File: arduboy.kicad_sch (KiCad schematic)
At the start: 59 parts, among them J1 Conn_01x06_Pin, J2 Conn_01x01_Pin, J3 Conn_01x01_Pin, J4 Conn_01x01_Pin, J5 Conn_01x01_Pin, J6 Conn_01x01_Pin, J7 Conn_01x01_Pin, SW1 POWER, SW2 LEFT, SW3 UP, SW4 DOWN, SW5 RIGHT, SW6 A, SW7 B, SW8 RESET, U1 ATmega32U4-A, U2 USBLC6-2SC6, U3 MCP73831-2-OT, U4 W25Q128JVS, Y1 16MHz

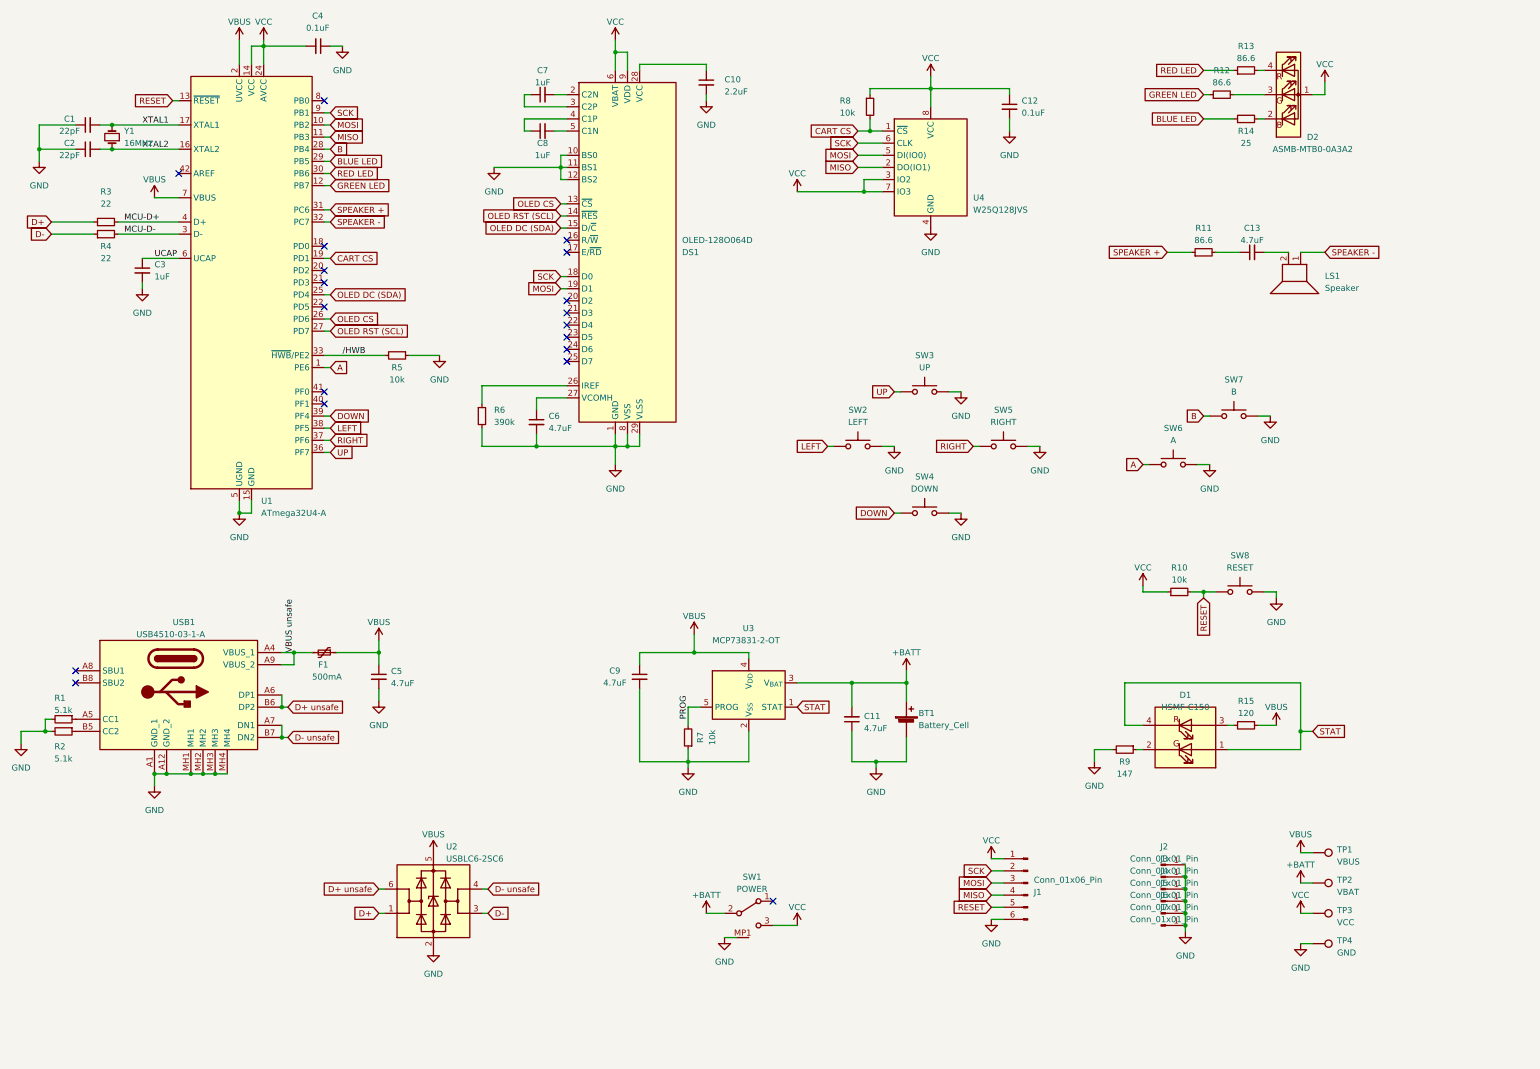
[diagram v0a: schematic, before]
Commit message: Add back silkscreen
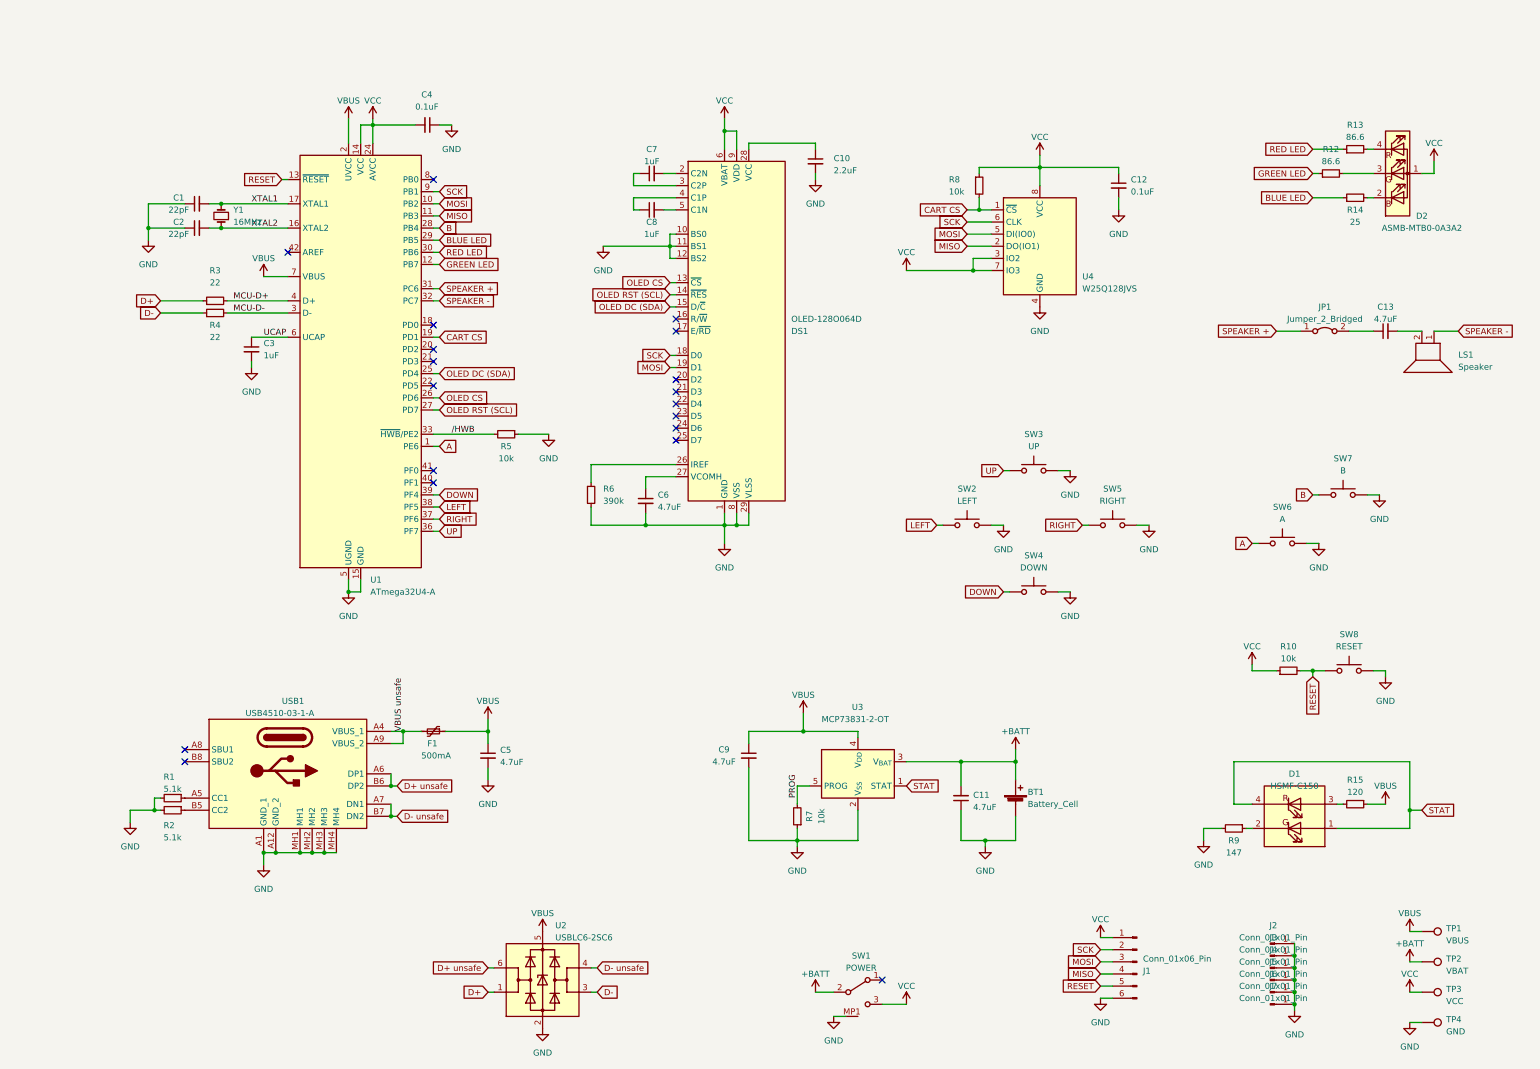
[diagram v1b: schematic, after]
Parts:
- removed R11: 86.6, arduboy:R_1210_3225Metric_Pad1.30x2.65mm_HandSolder with ref under the component, symbol Device:R_Small
- added JP1: Jumper_2_Bridged, arduboy:Jumper for SMD 1210 bridged, symbol Jumper:Jumper_2_Bridged
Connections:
- net SPEAKER +: now also JP1.1 (A)
- net at C13.1: now also JP1.2 (B)
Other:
- moved on the sheet: BT1, C1, C10, C11, C12, C13, C2, C3, C4, C5, C6, C7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

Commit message: Fix footprints to use 1210 according to selected components
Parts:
- C1, C10, C11, C12, C13, C2, C3, C4, C5, C6, C7, C8, C9: footprint arduboy:C_1210_3225Metric_Pad1.33x2.70mm_HandSolder ref under the component -> arduboy:C_1206_3216Metric_Pad1.33x1.80mm_HandSolder ref under the component
- JP1: footprint arduboy:Jumper for SMD 1210 bridged -> arduboy:Jumper for SMD 1206 bridged
- R1, R10, R12, R13, R14, R15, R2, R3, R4, R5, R6, R7, R8, R9: footprint arduboy:R_1210_3225Metric_Pad1.30x2.65mm_HandSolder with ref under the component -> arduboy:R_1206_3216Metric_Pad1.30x1.75mm_HandSolder with ref under the component
